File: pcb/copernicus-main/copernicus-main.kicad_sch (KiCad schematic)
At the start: 31 parts, among them J1 Screw_Terminal_01x02, J2 USB_C_14P, SW1 PWR_BTN, SW2 ESTOP, SW3 BOOT_SW, SW4 SW_DPST, U1 STM32F303CBTx, U2 SN65HVD230, U3 USBLC6-2SC6, U4 THVD1450D, U5 THVD1400D, Y1 16MHz

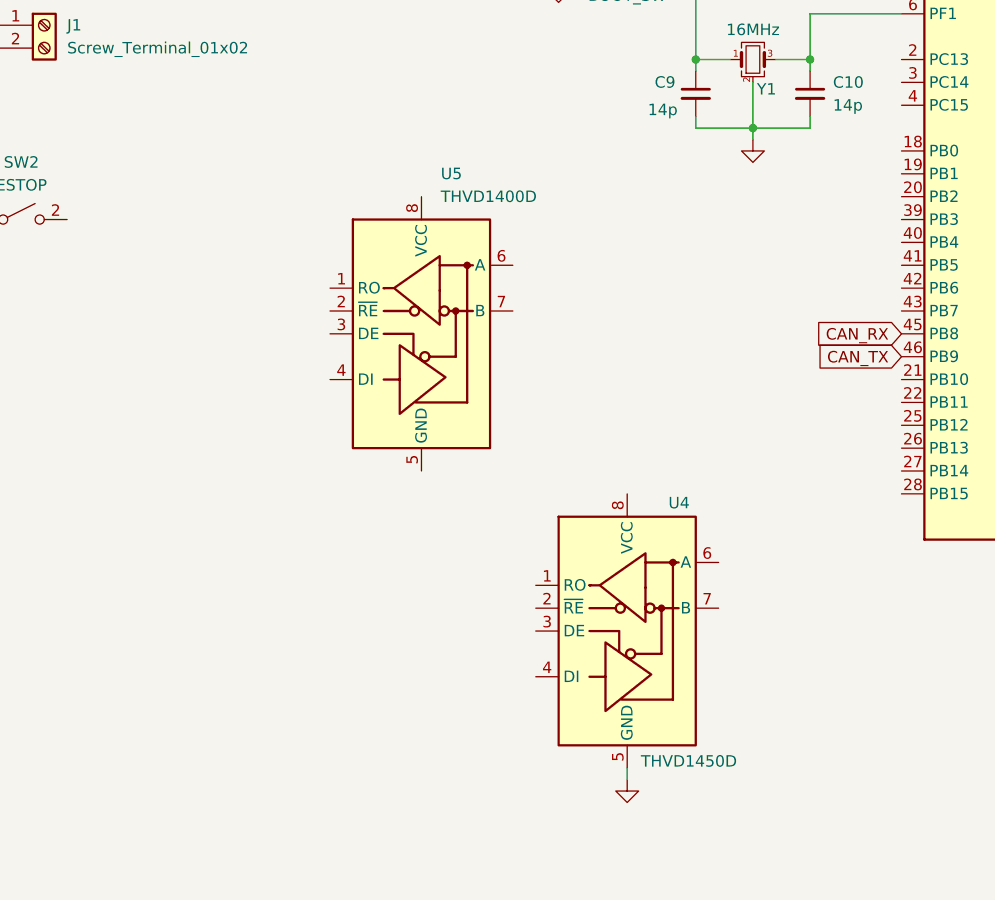
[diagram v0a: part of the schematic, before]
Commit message: commit
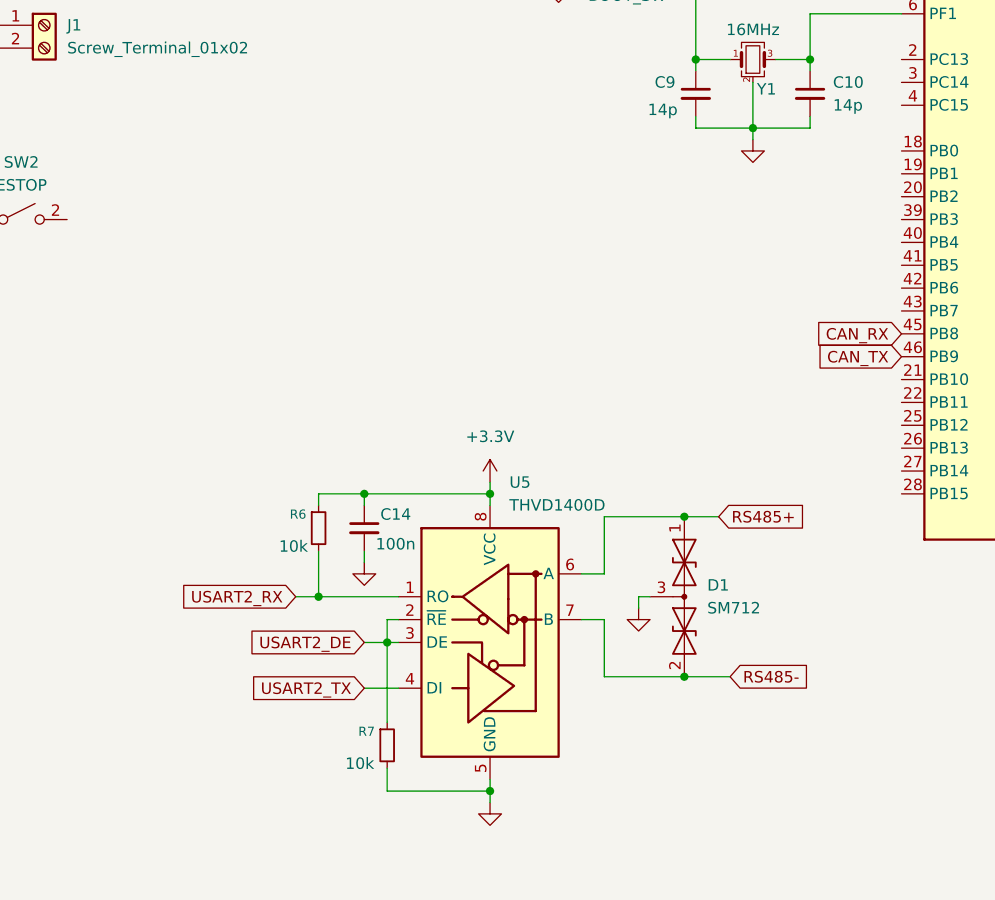
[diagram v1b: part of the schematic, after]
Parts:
- removed U4: THVD1450D, Package_SO:SOIC-8_3.9x4.9mm_P1.27mm, symbol Interface_UART:THVD1450D
- added C14: 100n, symbol Device:C_Small
- added D1: SM712, Package_TO_SOT_SMD:SOT-23, symbol Diode:SM712_SOT23
- added R6, R7: 10k, symbol Device:R_Small
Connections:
- net +3.3V: now also U5.8 (VCC), C14.1, R6.1
- net GND: now also U5.5 (GND), C14.2, D1.3 (common), R7.2
- net USART2_DE: now also U5.2 (~{RE}), U5.3 (DE), R7.1
- net USART2_RX: now also U5.1 (RO), R6.2
- net USART2_TX: now also U5.4 (DI)
- net RS485+: now reaches U5.6 (A)
- net RS485+: now also D1.1 (A1)
- net RS485-: now reaches U5.7 (B)
- net RS485-: now also D1.2 (A2)
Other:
- moved on the sheet: U5
